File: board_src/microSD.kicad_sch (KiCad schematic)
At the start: 7 parts, among them J12 112J-TDAR-R01, J14 Conn_01x07

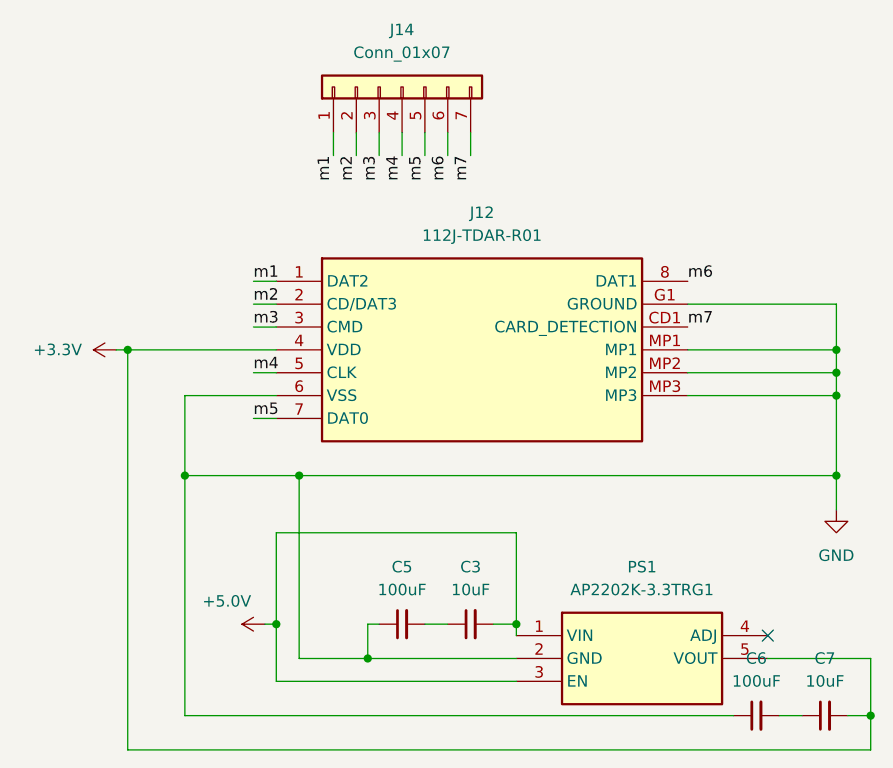
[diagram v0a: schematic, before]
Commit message: wersja z FT232RN
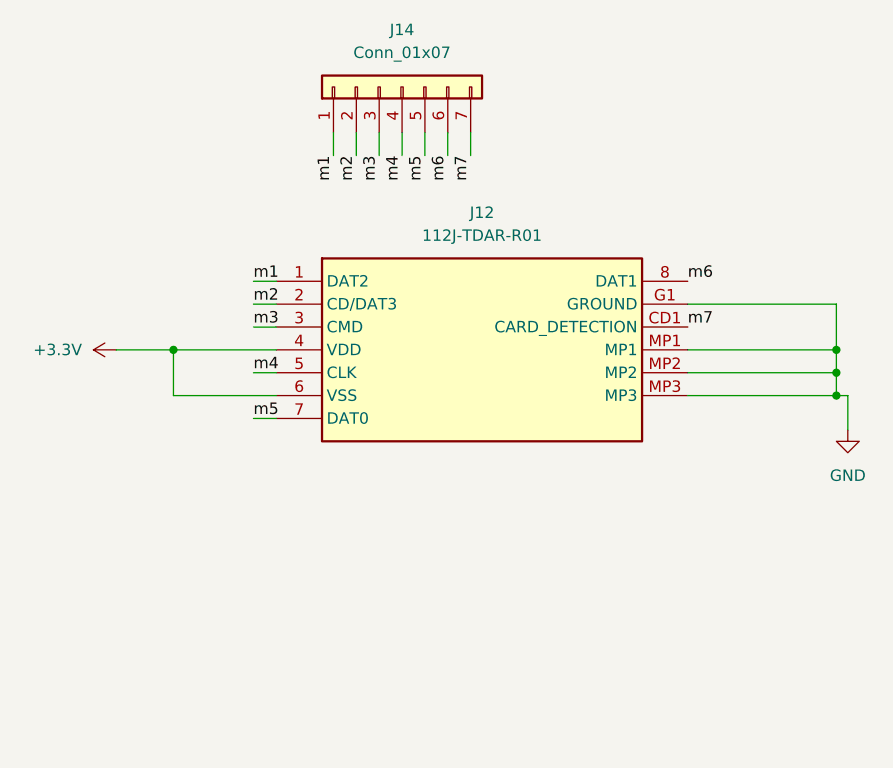
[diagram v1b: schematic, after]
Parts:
- removed C3, C7: 10uF, Capacitor_SMD:C_0201_0603Metric, symbol Device:C_Small
- removed C5, C6: 100uF, Capacitor_SMD:C_0201_0603Metric, symbol Device:C_Small
- removed PS1: AP2202K-3.3TRG1, footprints:SOT95P282X145-5N, symbol AP2202K-3_3TRG1:AP2202K-3.3TRG1
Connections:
- net +3.3V: now also J12.6 (VSS)
- net GND: no longer J12.6 (VSS)
- no-connect marks 1 -> 0
